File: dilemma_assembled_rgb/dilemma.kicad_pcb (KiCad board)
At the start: 2 copper layers, 134.1 x 110.3 mm, 122 parts, among them J1 USB_C_Receptacle_USB2.0, J102 Serial, J105 Conn_01x04_Female, J113 Cirque, J2 Conn_01x03_Female, J5 Conn_01x02, SW1 SW_Push, SW110 SW_SPST, SW2 SW_Push, SW3002 RotaryEncoder_Switch, U1 RP2040, U2 GD25Q80CEIGR, U3 XC6210B332MR-G, U4 USBLC6-2P6, Y1 Crystal_GND24

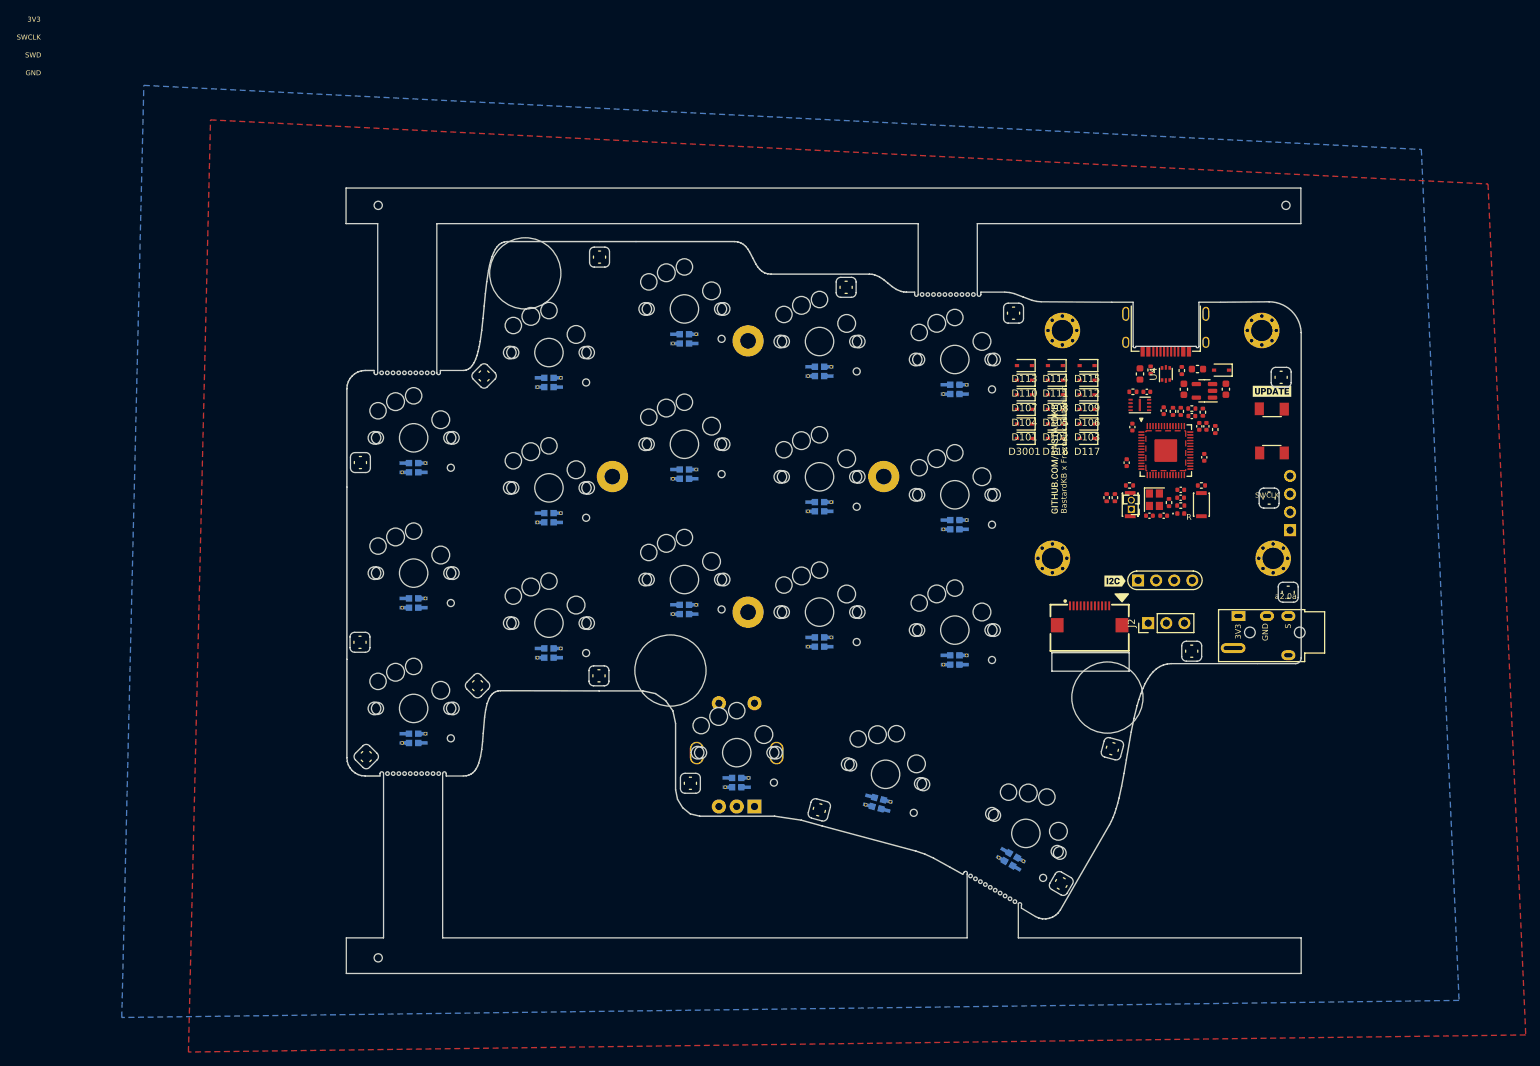
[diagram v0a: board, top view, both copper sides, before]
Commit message: edge cuts
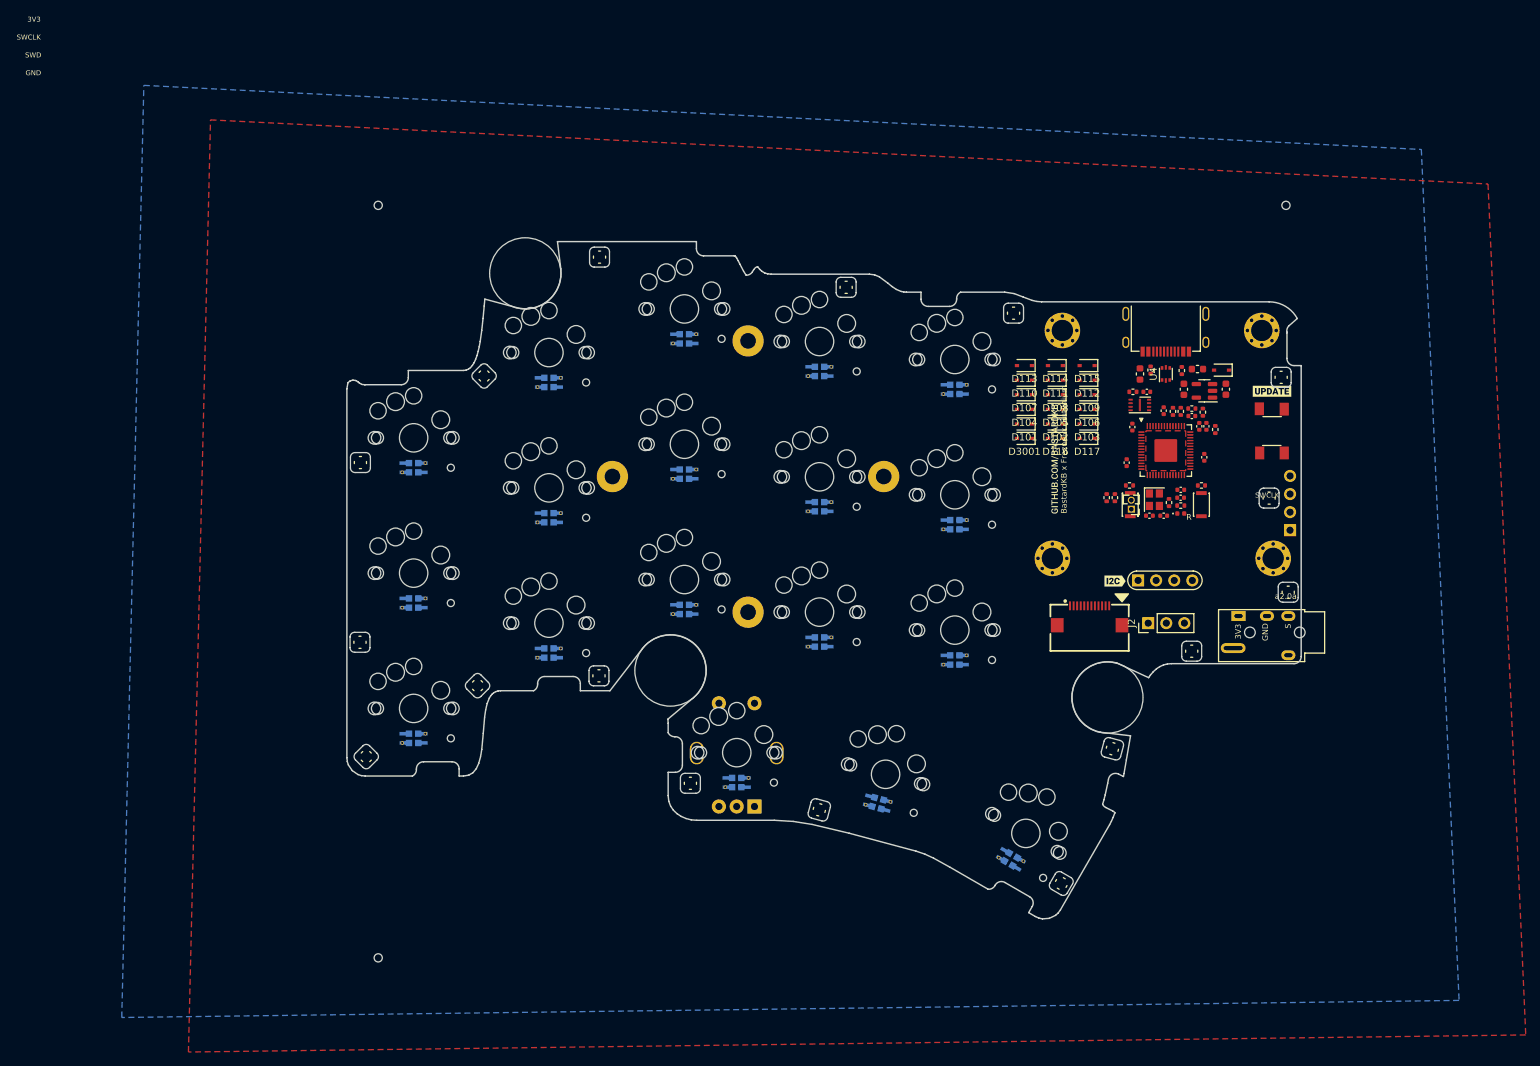
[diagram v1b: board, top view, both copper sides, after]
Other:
- board size 134.1 x 110.3 mm -> 134 x 95.1 mm
